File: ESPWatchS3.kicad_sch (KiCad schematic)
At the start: 114 parts, among them J1 OLED, J2 USB, J3 UART0, U1 ESP32-S3R8, U10 BD48KxxG, U2 EVA-M8Q-0, U3 BME280, U4 IS25LP128F-JKLE, U5 BQ27441-G1A, U6 BQ24075RGTR, U7 TPS631000DRLR, U8 AP3012, U9 NJG1143UA2-TE1, Y1 40MHz, Y2 32.768kHz, Y3 32.768kHz

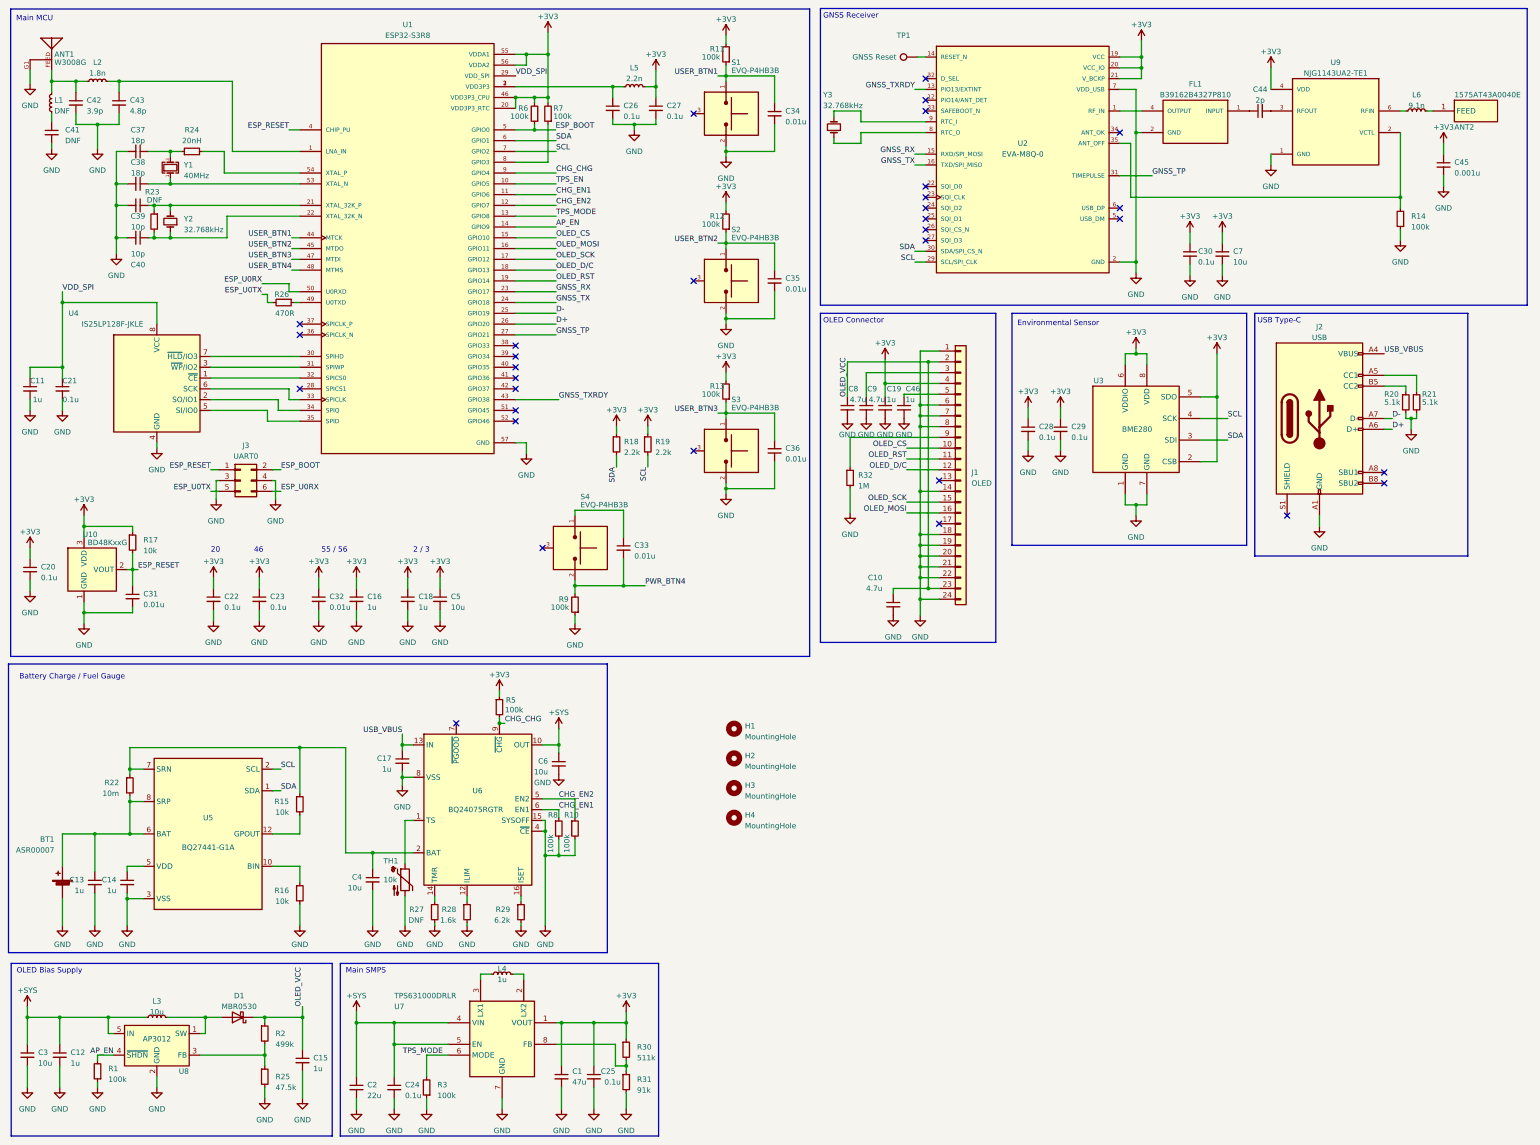
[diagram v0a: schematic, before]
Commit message: Library and schematic cleanup, revised designwork
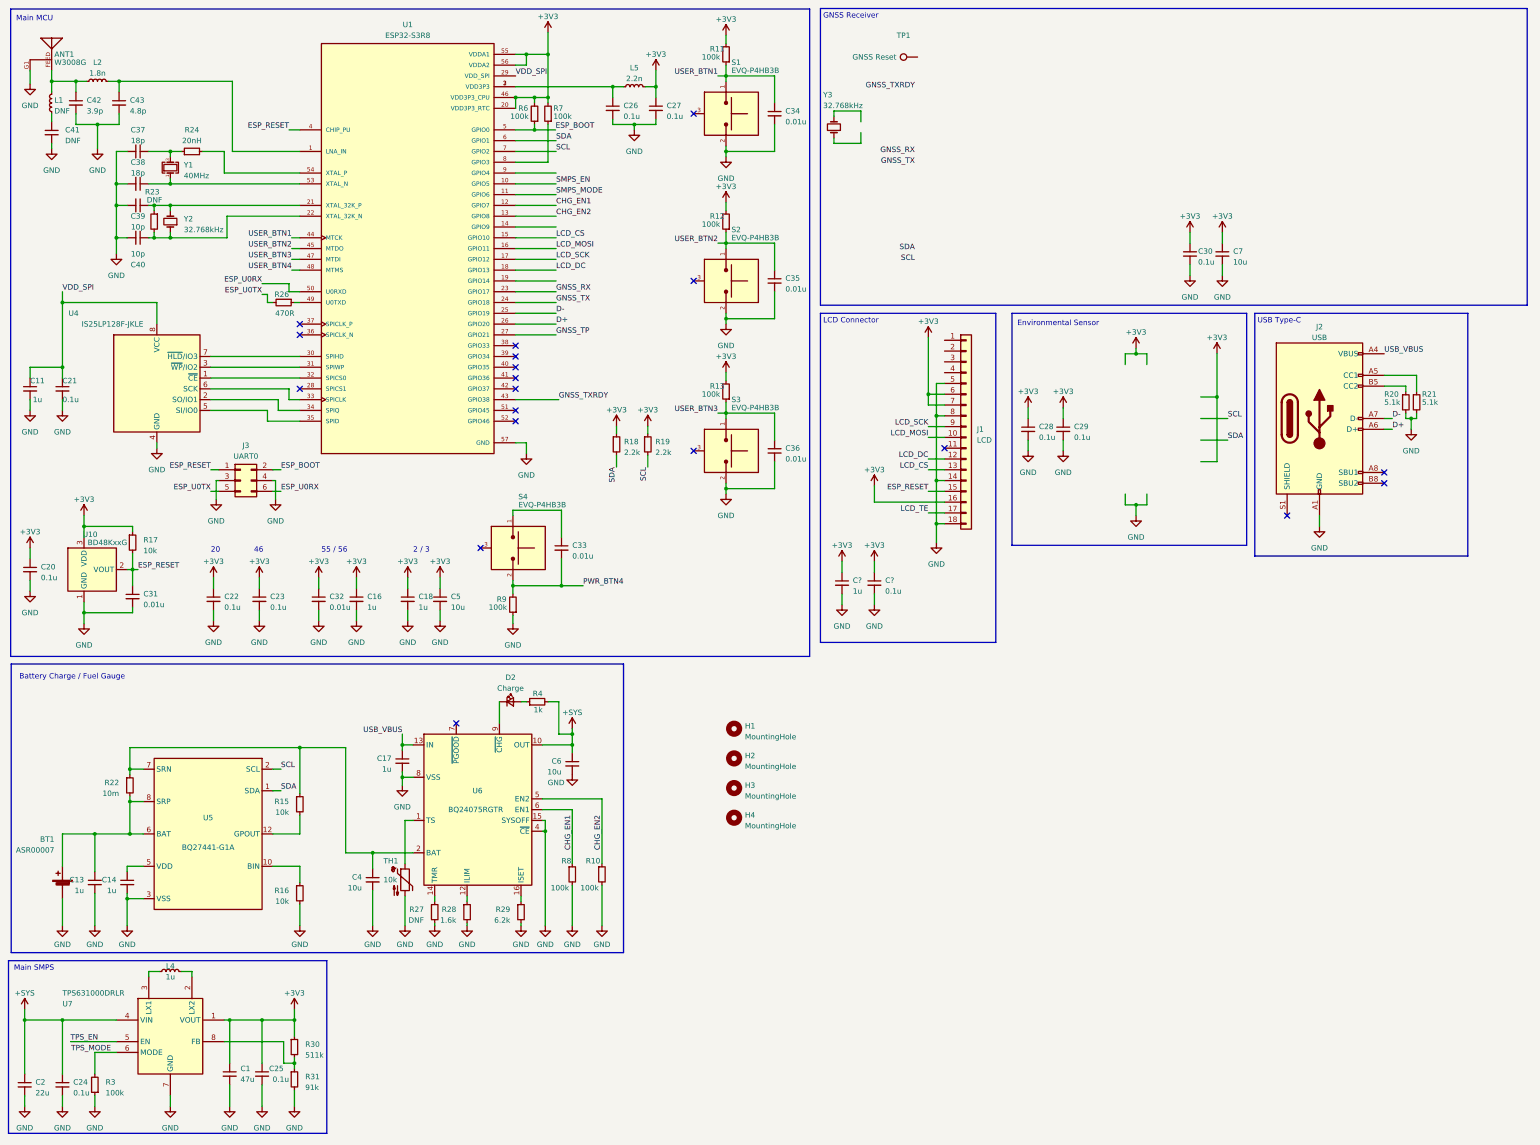
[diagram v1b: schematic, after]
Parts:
- removed ANT2: 1575AT43A0040E, WatchParts:1575AT43A0040E, symbol WatchParts:1575AT43A0040E
- removed C10, C8, C9: 4.7u, Capacitor_SMD:C_0603_1608Metric, symbol Device:C_Small
- removed C12, C15, C19, C46: 1u, Capacitor_SMD:C_0402_1005Metric, symbol Device:C_Small
- removed C3: 10u, Capacitor_SMD:C_0402_1005Metric, symbol Device:C_Small
- removed C44: 2p, Capacitor_SMD:C_0402_1005Metric, symbol Device:C_Small
- removed C45: 0.001u, Capacitor_SMD:C_0402_1005Metric, symbol Device:C_Small
- removed D1: MBR0530, Diode_SMD:D_SOD-123, symbol Diode:MBR0530
- removed FL1: B39162B4327P810, WatchParts:FIL_B39162B4327P810, symbol WatchParts:B39162B4327P810
- removed J1: OLED, WatchParts:CS050Z24GA0, symbol Connector_Generic:Conn_01x24
- removed L3: 10u, Inductor_SMD:L_1008_2520Metric, symbol Device:L_Small
- removed L6: 9.1n, Inductor_SMD:L_0402_1005Metric, symbol Device:L_Small
- removed R1, R14, R5: 100k, Resistor_SMD:R_0402_1005Metric, symbol Device:R_Small
- removed R2: 499k, Resistor_SMD:R_0402_1005Metric, symbol Device:R_Small
- removed R25: 47.5k, Resistor_SMD:R_0402_1005Metric, symbol Device:R_Small
- removed R32: 1M, Resistor_SMD:R_0402_1005Metric, symbol Device:R_Small
- removed U2: EVA-M8Q-0, WatchParts:LGA43R65P9X9_700X700X116, symbol WatchParts:EVA-M8Q-0
- removed U3: BME280, Package_LGA:Bosch_LGA-8_2.5x2.5mm_P0.65mm_ClockwisePinNumbering, symbol Sensor:BME280
- removed U8: AP3012, Package_TO_SOT_SMD:SOT-23-5, symbol Regulator_Switching:AP3012
- removed U9: NJG1143UA2-TE1, WatchParts:AMP_NJG1143UA2-TE1, symbol WatchParts:NJG1143UA2-TE1
- added C?: 1u, Capacitor_SMD:C_0402_1005Metric, symbol Device:C_Small
- added C?: 0.1u, Capacitor_SMD:C_0402_1005Metric, symbol Device:C_Small
- added D2: Charge, symbol Device:LED_Small
- added J1: LCD, symbol Connector_Generic:Conn_01x18
- added R4: 1k, Resistor_SMD:R_0402_1005Metric, symbol Device:R_Small
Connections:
- net +3V3: now also C?.1, C?.1, J1.16 (Pin_16), J1.6 (Pin_6), J1.7 (Pin_7)
- net +SYS: now also R4.2; no longer U7.5 (EN)
- net CHG_EN1: now also U1.12 (GPIO7); no longer U1.11 (GPIO6)
- net CHG_EN2: now also U1.13 (GPIO8); no longer U1.12 (GPIO7)
- net EP: now also C?.2, C?.2, J1.14 (Pin_14), J1.18 (Pin_18), J1.5 (Pin_5), J1.8 (Pin_8)
- net ESP_RESET: now also J1.15 (Pin_15)
- net TPS_EN: now also U7.5 (EN); no longer U1.10 (GPIO5)
- net TPS_MODE: no longer U1.13 (GPIO8)
- net AP_EN: no longer names the net of U1.14 (GPIO9)
- net CHG_CHG: no longer names the net of U6.9 (~{CHG})
- net CHG_CHG: now also D2.1 (K); no longer U1.9 (GPIO4)
- net OLED_CS renamed LCD_CS
- net LCD_CS: now also J1.13 (Pin_13)
- net OLED_D/C renamed LCD_DC
- net LCD_DC: now also J1.12 (Pin_12)
- net OLED_MOSI renamed LCD_MOSI
- net LCD_MOSI: now also J1.10 (Pin_10)
- net OLED_RST: no longer names the net of U1.19 (GPIO14)
- net OLED_SCK renamed LCD_SCK
- net LCD_SCK: now also J1.9 (Pin_9)
- new net: D2.2 (A), R4.1
- new net LCD_TE: J1.17 (Pin_17)
- new net SMPS_EN: U1.10 (GPIO5)
- new net SMPS_MODE: U1.11 (GPIO6)
- no-connect marks 32 -> 19
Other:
- note added: "LCD Connector"
- note removed: "OLED Bias Supply"
- note removed: "OLED Connector"
- moved on the sheet: C1, C2, C24, C25, C29, C33, C6, L4, R10, R3, R30, R31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
